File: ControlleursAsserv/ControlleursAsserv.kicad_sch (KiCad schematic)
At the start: 42 parts, among them J1 I2C1_5, J2 I2C2_5, J3 CAN1, J4 CAN2, J5 In App Prog, J6 DEBUG, SW1 RESET, SW2 BOOT0, U1 STM32G474RETx, U2 AMS1117-3.3, U3 MCP2558FD-xSN, Y1 16MHz

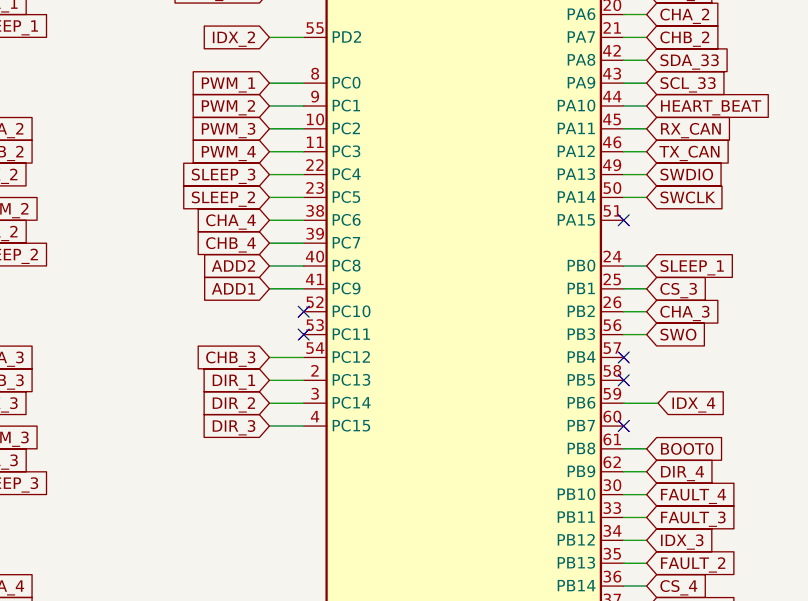
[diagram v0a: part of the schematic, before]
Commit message: Init routing
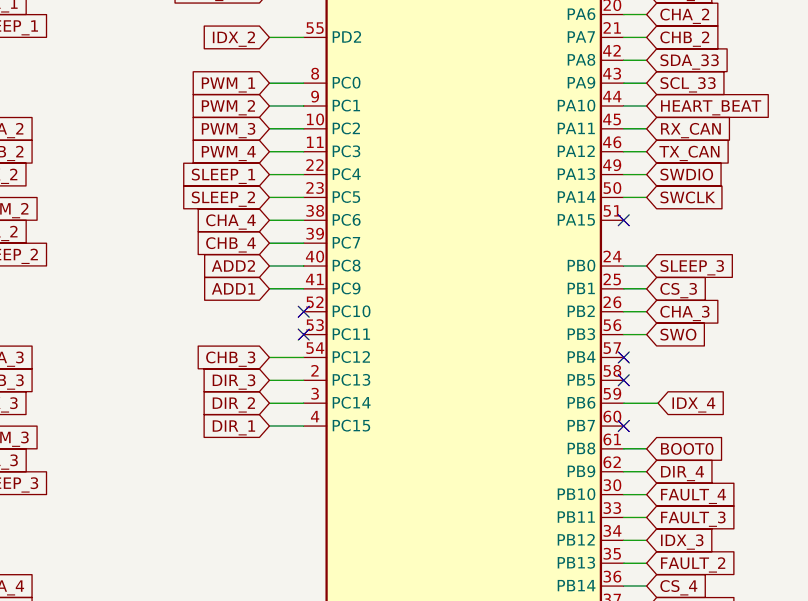
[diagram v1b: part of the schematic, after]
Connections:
- net DIR_1: now also U1.4 (PC15); no longer U1.2 (PC13)
- net DIR_3: now also U1.2 (PC13); no longer U1.4 (PC15)
- net SLEEP_1: now also U1.22 (PC4); no longer U1.24 (PB0)
- net SLEEP_3: now also U1.24 (PB0); no longer U1.22 (PC4)
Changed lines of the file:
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@@
     )
   )
-  (global_label "SLEEP_3" (shape input) (at 213.36 83.82 180) (fields_autoplaced)
-    (effects (font (size 1.27 1.27)) (justify right))
-    (property "Intersheetrefs" "${INTERSHEET_REFS}" (at 202.3921 83.82 0)
-      (effects (font (size 1.27 1.27)) (justify right) hide)
+  (global_label "SLEEP_3" (shape input) (at 255.27 93.98 0) (fields_autoplaced)
+    (effects (font (size 1.27 1.27)) (justify left))
+    (property "Intersheetrefs" "${INTERSHEET_REFS}" (at 266.2379 93.98 0)
+      (effects (font (size 1.27 1.27)) (justify left) hide)
     )
   )
@@
     )
   )
-  (global_label "SLEEP_1" (shape input) (at 255.27 93.98 0) (fields_autoplaced)
-    (effects (font (size 1.27 1.27)) (justify left))
-    (property "Intersheetrefs" "${INTERSHEET_REFS}" (at 266.2379 93.98 0)
-      (effects (font (size 1.27 1.27)) (justify left) hide)
+  (global_label "SLEEP_1" (shape input) (at 213.36 83.82 180) (fields_autoplaced)
+    (effects (font (size 1.27 1.27)) (justify right))
+    (property "Intersheetrefs" "${INTERSHEET_REFS}" (at 202.3921 83.82 0)
+      (effects (font (size 1.27 1.27)) (justify right) hide)
     )
   )
@@
     )
   )
-  (global_label "DIR_3" (shape input) (at 213.36 111.76 180) (fields_autoplaced)
+  (global_label "DIR_3" (shape input) (at 213.36 106.68 180) (fields_autoplaced)
     (effects (font (size 1.27 1.27)) (justify right))
-    (property "Intersheetrefs" "${INTERSHEET_REFS}" (at 205.0529 111.76 0)
+    (property "Intersheetrefs" "${INTERSHEET_REFS}" (at 205.0529 106.68 0)
       (effects (font (size 1.27 1.27)) (justify right) hide)
     )
@@
     )
   )
-  (global_label "DIR_1" (shape input) (at 213.36 106.68 180) (fields_autoplaced)
+  (global_label "DIR_1" (shape input) (at 213.36 111.76 180) (fields_autoplaced)
     (effects (font (size 1.27 1.27)) (justify right))
-    (property "Intersheetrefs" "${INTERSHEET_REFS}" (at 205.0529 106.68 0)
+    (property "Intersheetrefs" "${INTERSHEET_REFS}" (at 205.0529 111.76 0)
       (effects (font (size 1.27 1.27)) (justify right) hide)
     )

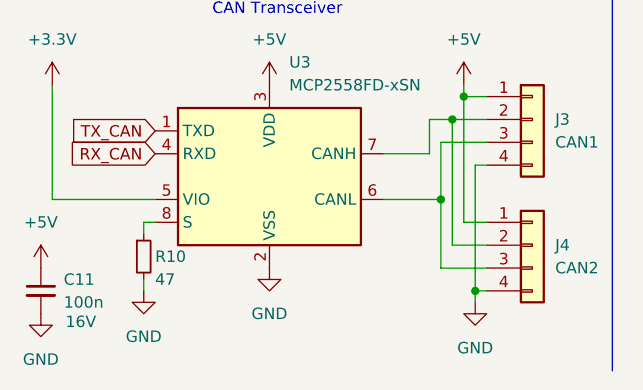
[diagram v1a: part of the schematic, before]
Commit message: Finish Controller Asserv
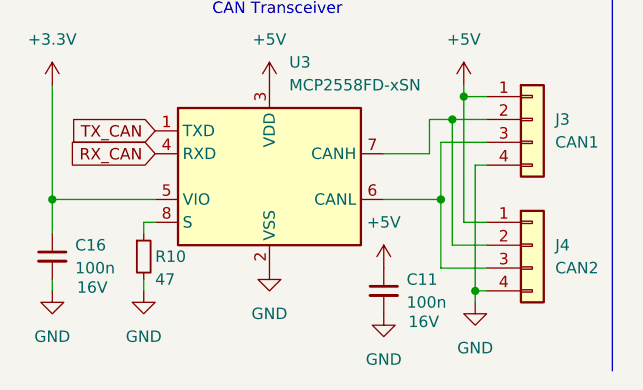
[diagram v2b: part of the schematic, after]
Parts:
- added C16: 100n, Capacitor_SMD:C_0402_1005Metric_Pad0.74x0.62mm_HandSolder, symbol Device:C_Small
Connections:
- net +3.3V: now also C16.1
- net GND: now also C16.2
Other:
- moved on the sheet: C11
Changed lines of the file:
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@@
   (junction (at 41.91 53.34) (diameter 0) (color 0 0 0 0)
+  )
+  (junction (at 16.51 177.8) (diameter 0) (color 0 0 0 0)
   )
   (junction (at 33.02 124.46) (diameter 0) (color 0 0 0 0)
@@
     (stroke (width 0) (type default))
   )
+  (wire (pts (xy 16.51 177.8) (xy 16.51 181.61))
+    (stroke (width 0) (type default))
+  )
   (wire (pts (xy 87.63 21.59) (xy 77.47 21.59))
     (stroke (width 0) (type default))
@@
   )
   (wire (pts (xy 64.77 171.45) (xy 59.69 171.45))
+    (stroke (width 0) (type default))
+  )
+  (wire (pts (xy 16.51 186.69) (xy 16.51 187.96))
     (stroke (width 0) (type default))
   )
@@
     )
   )
-  (symbol (lib_id "power:+5V") (at 15.24 185.42 0) (unit 1)
-    (in_bom yes) (on_board yes) (dnp no) (fields_autoplaced)
-    (property "Reference" "#PWR033" (at 15.24 189.23 0)
-      (effects (font (size 1.27 1.27)) hide)
-    )
-    (property "Value" "+5V" (at 15.24 180.34 0)
-      (effects (font (size 1.27 1.27)))
-    )
-    (property "Footprint" "" (at 15.24 185.42 0)
-      (effects (font (size 1.27 1.27)) hide)
-    )
-    (property "Datasheet" "" (at 15.24 185.42 0)
+  (symbol (lib_id "power:+5V") (at 53.34 185.42 0) (unit 1)
+    (in_bom yes) (on_board yes) (dnp no) (fields_autoplaced)
+    (property "Reference" "#PWR033" (at 53.34 189.23 0)
+      (effects (font (size 1.27 1.27)) hide)
+    )
+    (property "Value" "+5V" (at 53.34 180.34 0)
+      (effects (font (size 1.27 1.27)))
+    )
+    (property "Footprint" "" (at 53.34 185.42 0)
+      (effects (font (size 1.27 1.27)) hide)
+    )
+    (property "Datasheet" "" (at 53.34 185.42 0)
       (effects (font (size 1.27 1.27)) hide)
     )
@@
     )
   )
-  (symbol (lib_id "power:GND") (at 15.24 190.5 0) (unit 1)
-    (in_bom yes) (on_board yes) (dnp no) (fields_autoplaced)
-    (property "Reference" "#PWR034" (at 15.24 196.85 0)
-      (effects (font (size 1.27 1.27)) hide)
-    )
-    (property "Value" "GND" (at 15.24 195.58 0)
-      (effects (font (size 1.27 1.27)))
-    )
-    (property "Footprint" "" (at 15.24 190.5 0)
-      (effects (font (size 1.27 1.27)) hide)
-    )
-    (property "Datasheet" "" (at 15.24 190.5 0)
+  (symbol (lib_id "power:GND") (at 53.34 190.5 0) (unit 1)
+    (in_bom yes) (on_board yes) (dnp no) (fields_autoplaced)
+    (property "Reference" "#PWR034" (at 53.34 196.85 0)
+      (effects (font (size 1.27 1.27)) hide)
+    )
+    (property "Value" "GND" (at 53.34 195.58 0)
+      (effects (font (size 1.27 1.27)))
+    )
+    (property "Footprint" "" (at 53.34 190.5 0)
+      (effects (font (size 1.27 1.27)) hide)
+    )
+    (property "Datasheet" "" (at 53.34 190.5 0)
       (effects (font (size 1.27 1.27)) hide)
     )
@@
     )
   )
-  (symbol (lib_id "Device:C_Small") (at 15.24 187.96 0) (unit 1)
+  (symbol (lib_id "Device:C_Small") (at 53.34 187.96 0) (unit 1)
     (in_bom yes) (on_board yes) (dnp no)
-    (property "Reference" "C11" (at 17.78 186.6963 0)
-      (effects (font (size 1.27 1.27)) (justify left))
-    )
-    (property "Value" "100n" (at 17.78 189.2363 0)
-      (effects (font (size 1.27 1.27)) (justify left))
-    )
-    (property "Footprint" "Capacitor_SMD:C_0402_1005Metric_Pad0.74x0.62mm_HandSolder" (at 15.24 187.96 0)
-      (effects (font (size 1.27 1.27)) hide)
-    )
-    (property "Datasheet" "~" (at 15.24 187.96 0)
-      (effects (font (size 1.27 1.27)) hide)
-    )
-    (property "JLCPCB BOM" "" (at 15.24 187.96 0)
-      (effects (font (size 1.27 1.27)) hide)
-    )
-    (property "LCSC Part" "C1525" (at 15.24 187.96 0)
-      (effects (font (size 1.27 1.27)) hide)
-    )
-    (property "Tension" "16V" (at 19.685 191.389 0)
+    (property "Reference" "C11" (at 55.88 186.6963 0)
+      (effects (font (size 1.27 1.27)) (justify left))
+    )
+    (property "Value" "100n" (at 55.88 189.2363 0)
+      (effects (font (size 1.27 1.27)) (justify left))
+    )
+    (property "Footprint" "Capacitor_SMD:C_0402_1005Metric_Pad0.74x0.62mm_HandSolder" (at 53.34 187.96 0)
+      (effects (font (size 1.27 1.27)) hide)
+    )
+    (property "Datasheet" "~" (at 53.34 187.96 0)
+      (effects (font (size 1.27 1.27)) hide)
+    )
+    (property "JLCPCB BOM" "" (at 53.34 187.96 0)
+      (effects (font (size 1.27 1.27)) hide)
+    )
+    (property "LCSC Part" "C1525" (at 53.34 187.96 0)
+      (effects (font (size 1.27 1.27)) hide)
+    )
+    (property "Tension" "16V" (at 57.785 191.389 0)
       (effects (font (size 1.27 1.27)))
     )
@@
     )
   )
+  (symbol (lib_id "Device:C_Small") (at 16.51 184.15 0) (unit 1)
+    (in_bom yes) (on_board yes) (dnp no)
+    (property "Reference" "C16" (at 19.05 182.8863 0)
+      (effects (font (size 1.27 1.27)) (justify left))
+    )
+    (property "Value" "100n" (at 19.05 185.4263 0)
+      (effects (font (size 1.27 1.27)) (justify left))
+    )
+    (property "Footprint" "Capacitor_SMD:C_0402_1005Metric_Pad0.74x0.62mm_HandSolder" (at 16.51 184.15 0)
+      (effects (font (size 1.27 1.27)) hide)
+    )
+    (property "Datasheet" "~" (at 16.51 184.15 0)
+      (effects (font (size 1.27 1.27)) hide)
+    )
+    (property "JLCPCB BOM" "" (at 16.51 184.15 0)
+      (effects (font (size 1.27 1.27)) hide)
+    )
+    (property "LCSC Part" "C1525" (at 16.51 184.15 0)
+      (effects (font (size 1.27 1.27)) hide)
+    )
+    (property "Tension" "16V" (at 20.955 187.579 0)
+      (effects (font (size 1.27 1.27)))
+    )
+    (pin "1")
+    (pin "2")
+    (instances
+      (project "ControlleursAsserv"
+        (path "/c83bc042-587c-48f9-abdb-41233c8ec938"
+          (reference "C16") (unit 1)
+        )
+      )
+    )
+  )
   (symbol (lib_id "power:GND") (at 41.91 60.96 0) (unit 1)
     (in_bom yes) (on_board yes) (dnp no) (fields_autoplaced)
@@
         )
       )
+    )
+  )
+  (symbol (lib_id "power:GND") (at 16.51 187.96 0) (unit 1)
+    (in_bom yes) (on_board yes) (dnp no) (fields_autoplaced)
+    (property "Reference" "#PWR060" (at 16.51 194.31 0)
+      (effects (font (size 1.27 1.27)) hide)
+    )
+    (property "Value" "GND" (at 16.51 193.04 0)
+      (effects (font (size 1.27 1.27)))
+    )
+    (property "Footprint" "" (at 16.51 187.96 0)
+      (effects (font (size 1.27 1.27)) hide)
+    )
+    (property "Datasheet" "" (at 16.51 187.96 0)
+      (effects (font (size 1.27 1.27)) hide)
+    )
+    (pin "1")
+    (instances
+      (project "ControlleursAsserv"
+        (path "/c83bc042-587c-48f9-abdb-41233c8ec938"
+          (reference "#PWR060") (unit 1)
+        )
+      )
